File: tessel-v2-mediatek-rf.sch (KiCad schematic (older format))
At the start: 43 parts, among them J501 CONN_01X01, J502 CONN_01X01, T501 2450BL15B100, T502 2450BL15B100, U201 MT7620N

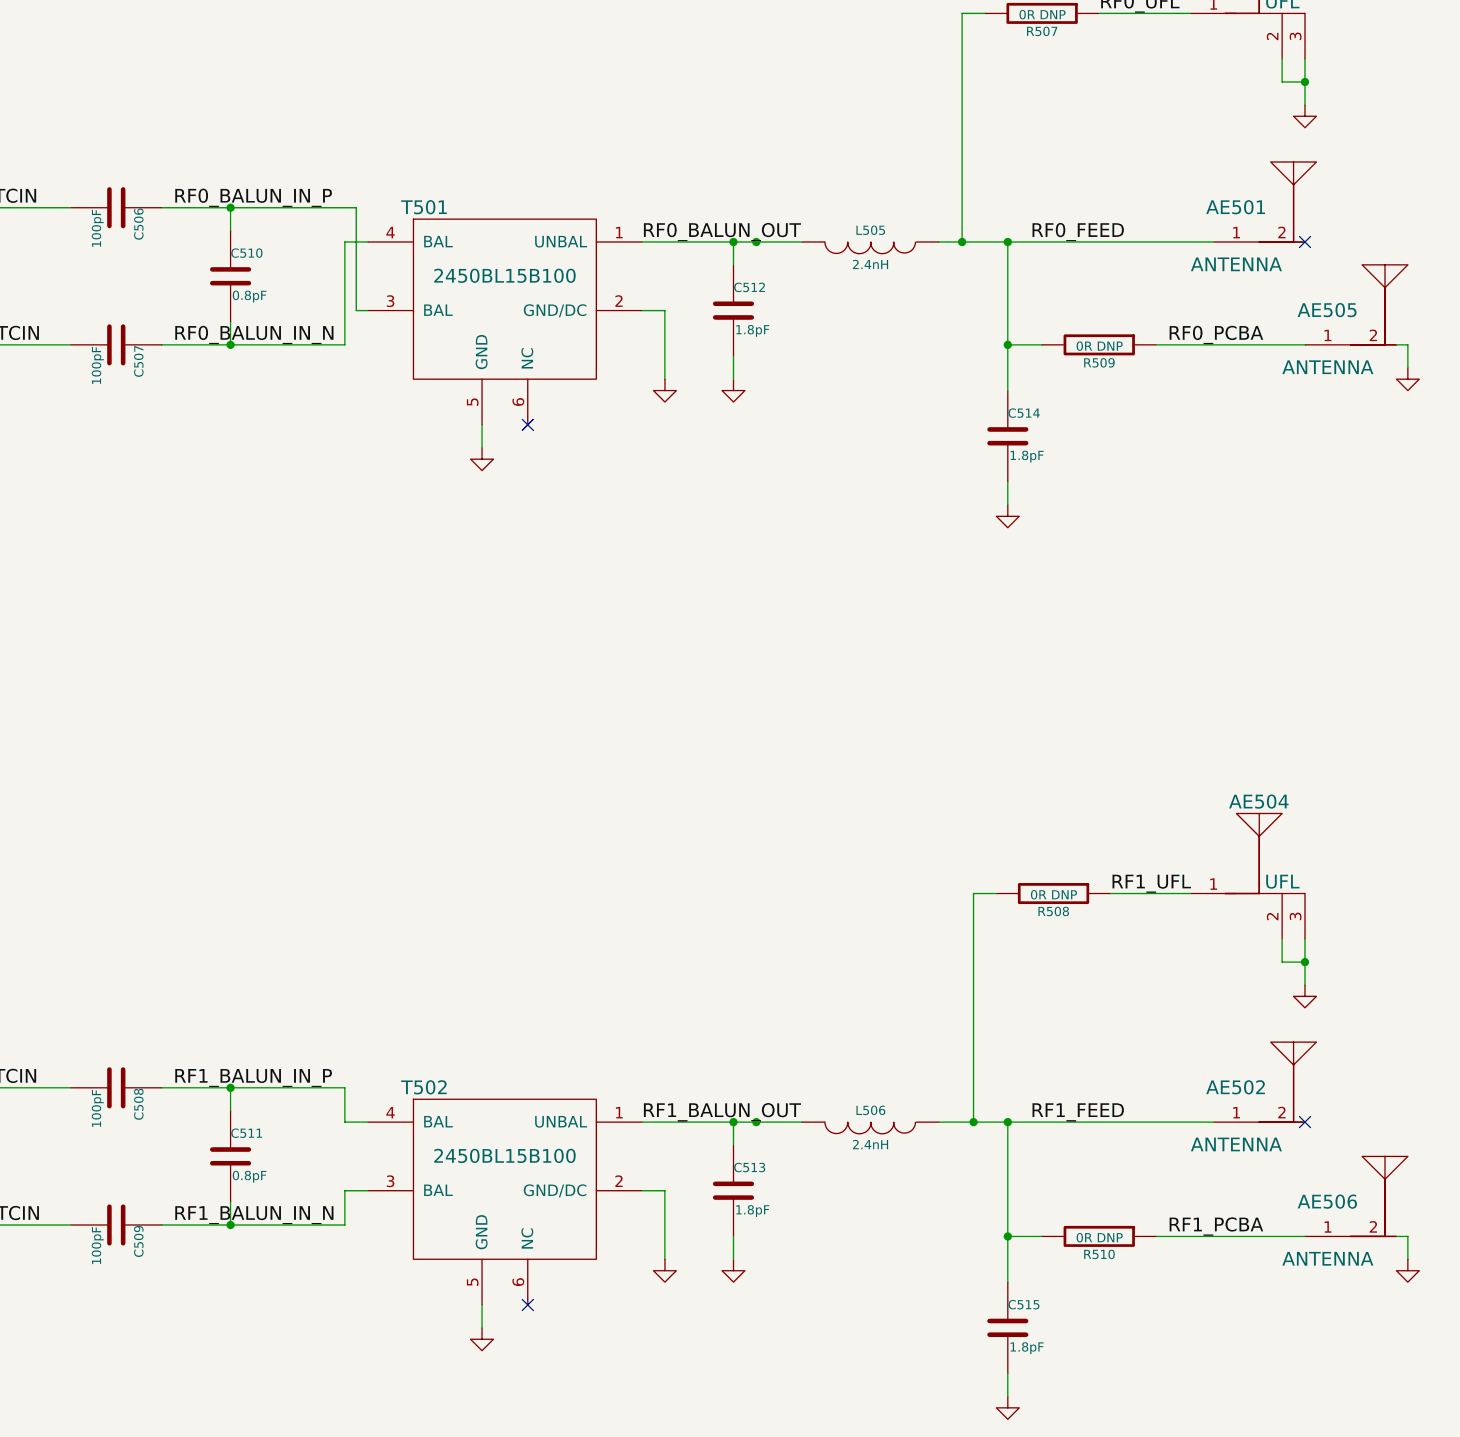
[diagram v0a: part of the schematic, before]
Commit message: pushing for jia
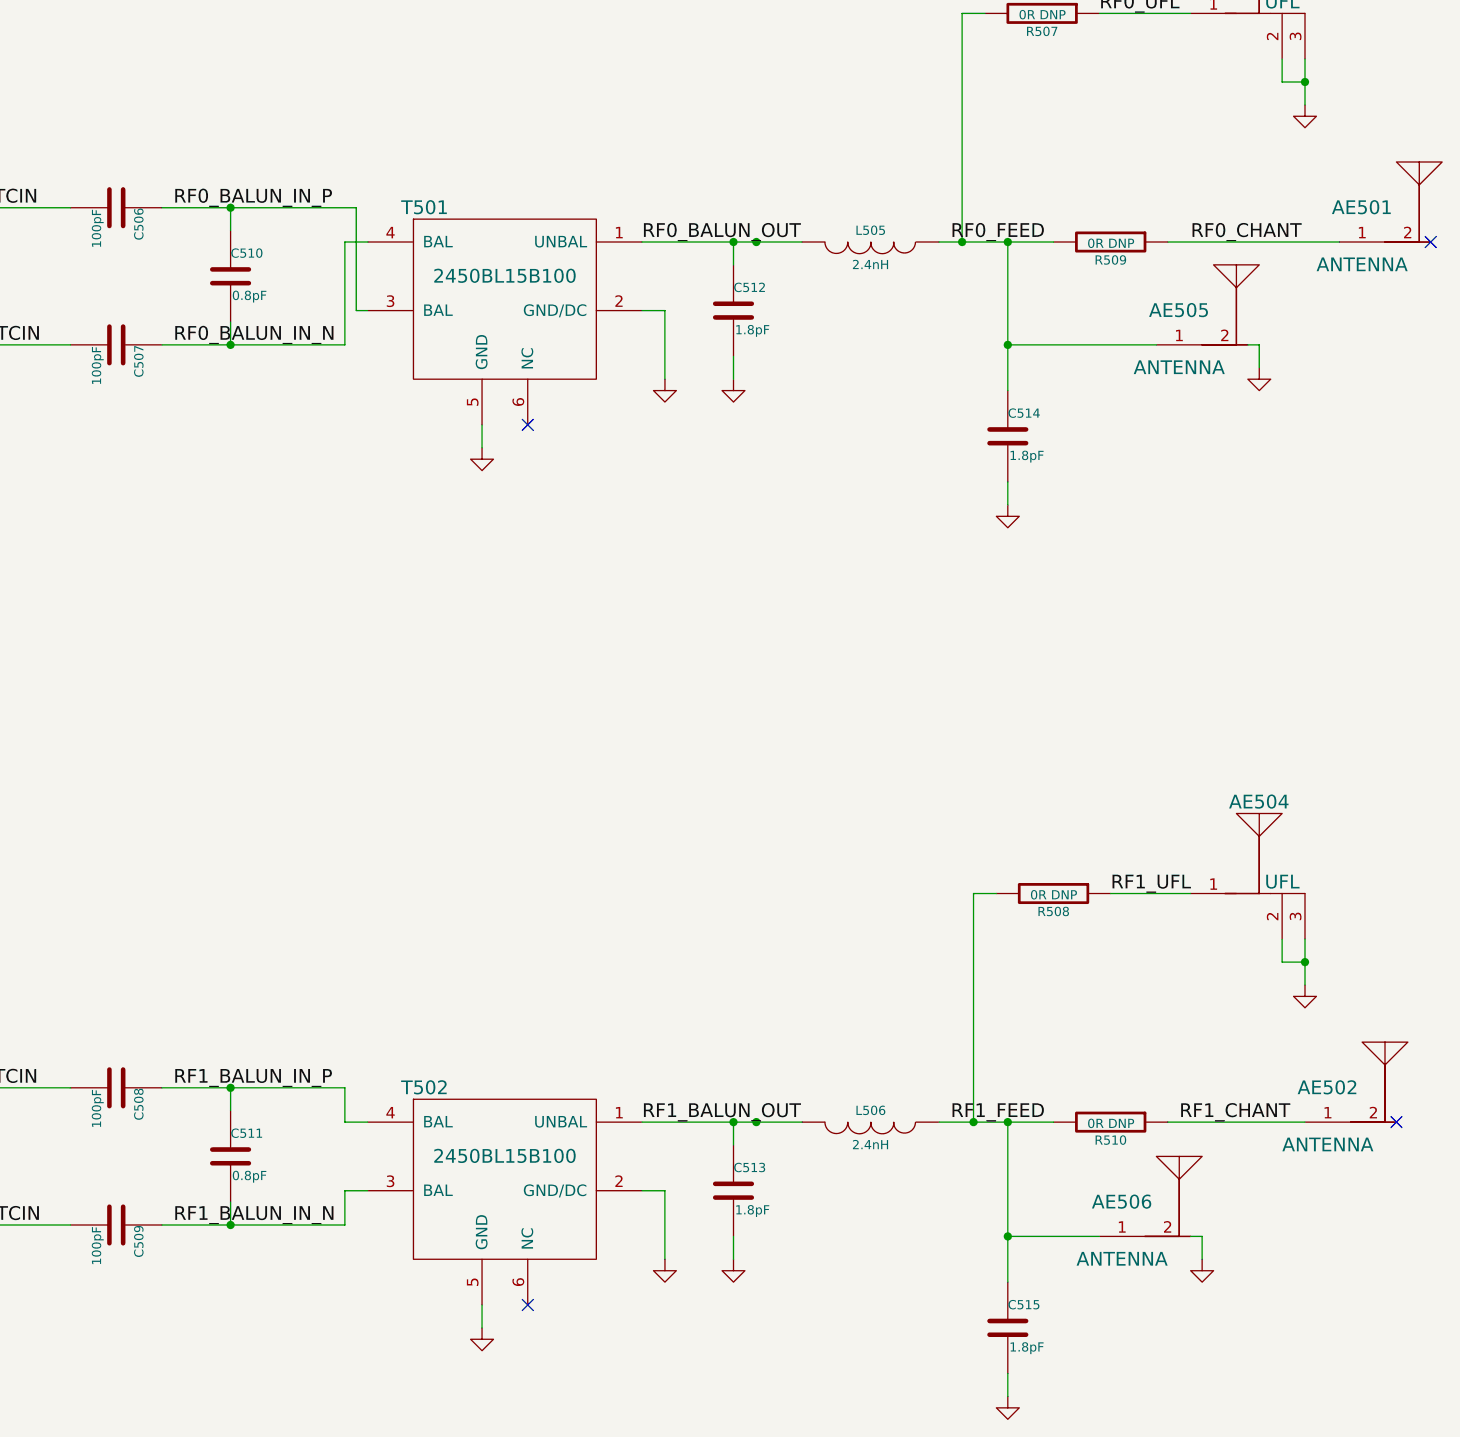
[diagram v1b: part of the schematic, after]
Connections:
- net RF0_FEED: now also AE505.1; no longer AE501.1
- net RF1_FEED: now also AE506.1; no longer AE502.1
- net RF0_PCBA renamed RF0_CHANT
- net RF0_CHANT: now also AE501.1; no longer AE505.1
- net RF1_PCBA renamed RF1_CHANT
- net RF1_CHANT: now also AE502.1; no longer AE506.1
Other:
- moved on the sheet: AE501, AE502, AE505, AE506, R509, R510

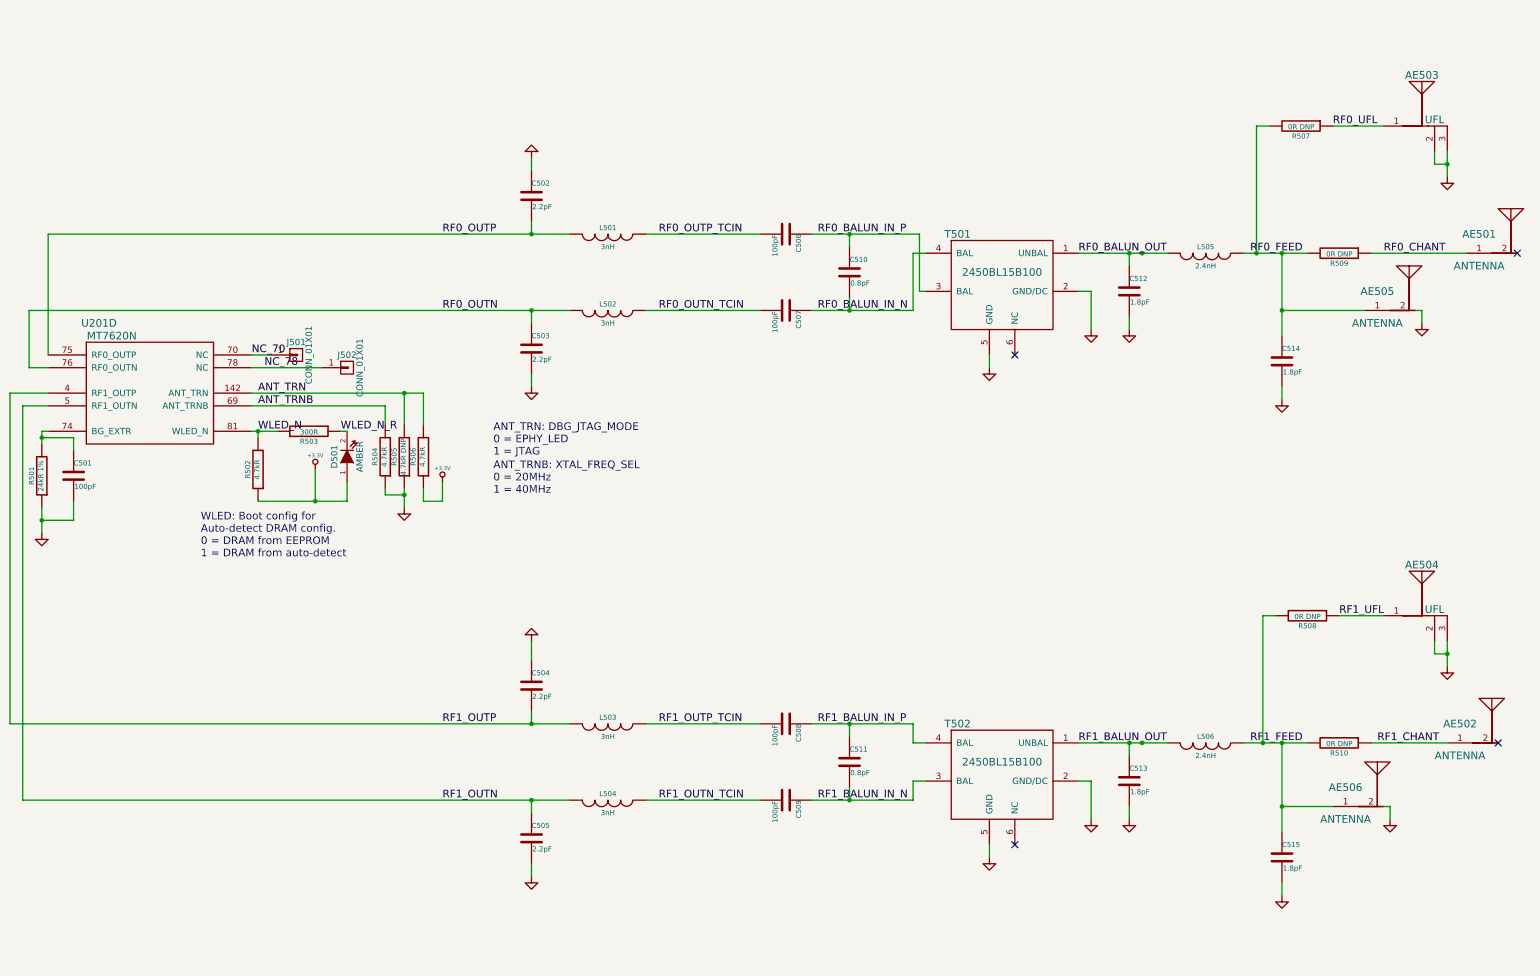
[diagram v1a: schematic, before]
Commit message: post-schematic review. changes in.
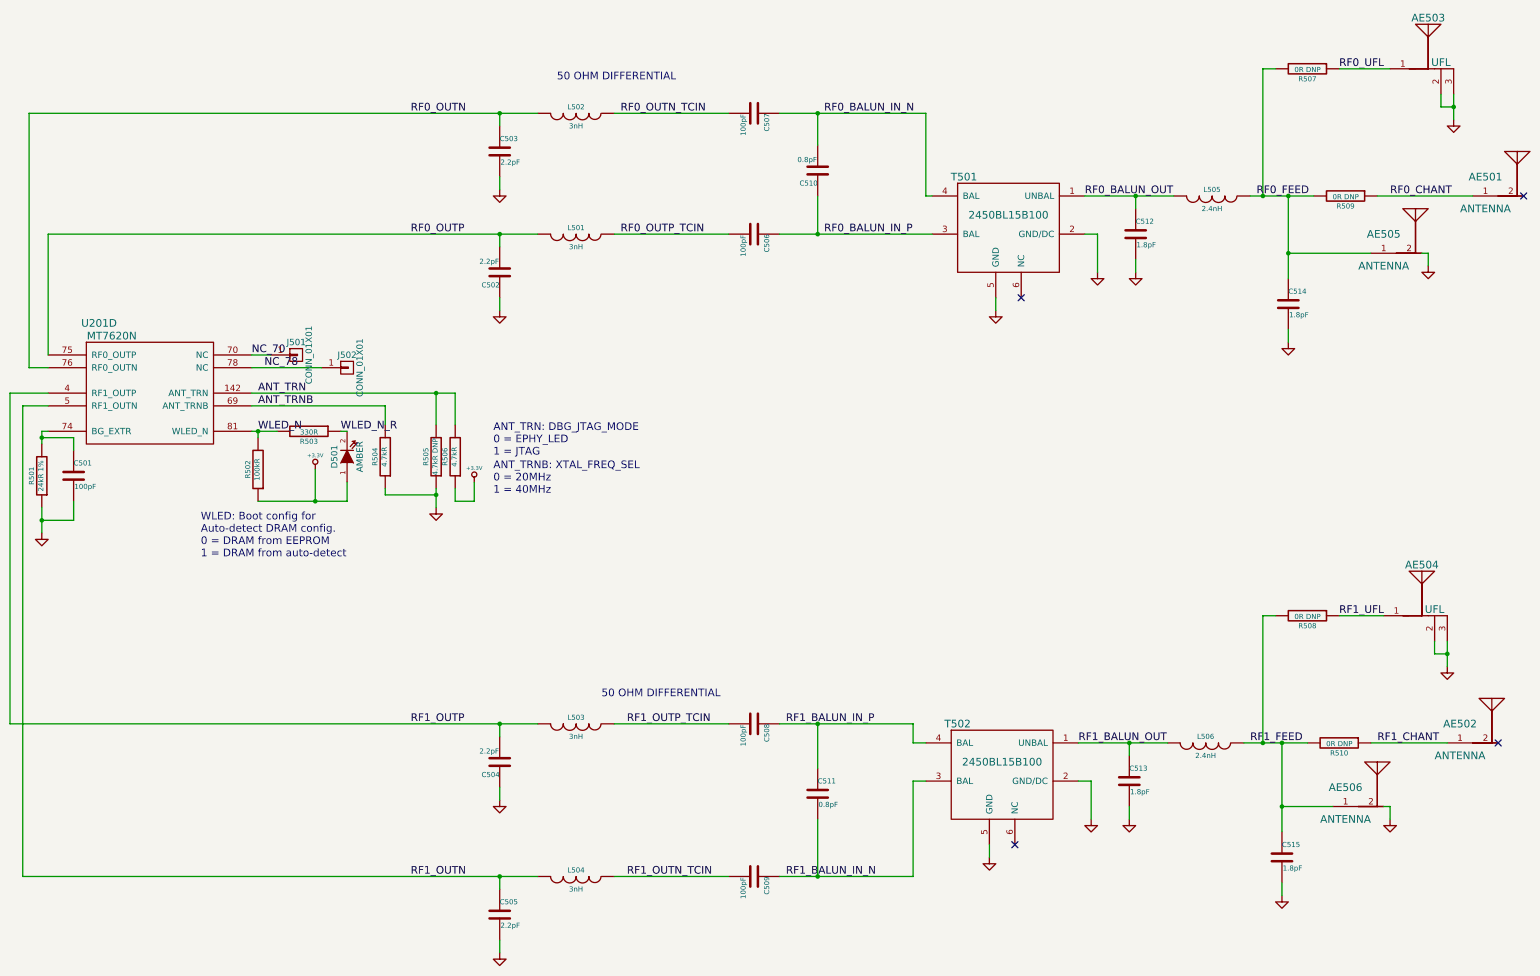
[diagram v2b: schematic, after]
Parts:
- R502: value 4.7kR -> 100kR
- R503: value 300R -> 330R
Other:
- note added: "50 OHM DIFFERENTIAL"
- moved on the sheet: AE501, AE503, AE505, C502, C503, C504, C505, C506, C507, C508, C509, C510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
